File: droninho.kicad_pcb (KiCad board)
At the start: 2 copper layers, 26 x 49 mm, 19 parts, among them J1 M1, J2 M1, J3 M1, J4 M1, J5 Conn_01x02_Pin, Q1 SI2300, Q2 SI2300, Q3 SI2300, Q4 SI2300, U1 ESP32 Dev Kit, U2 MPU9250/6500

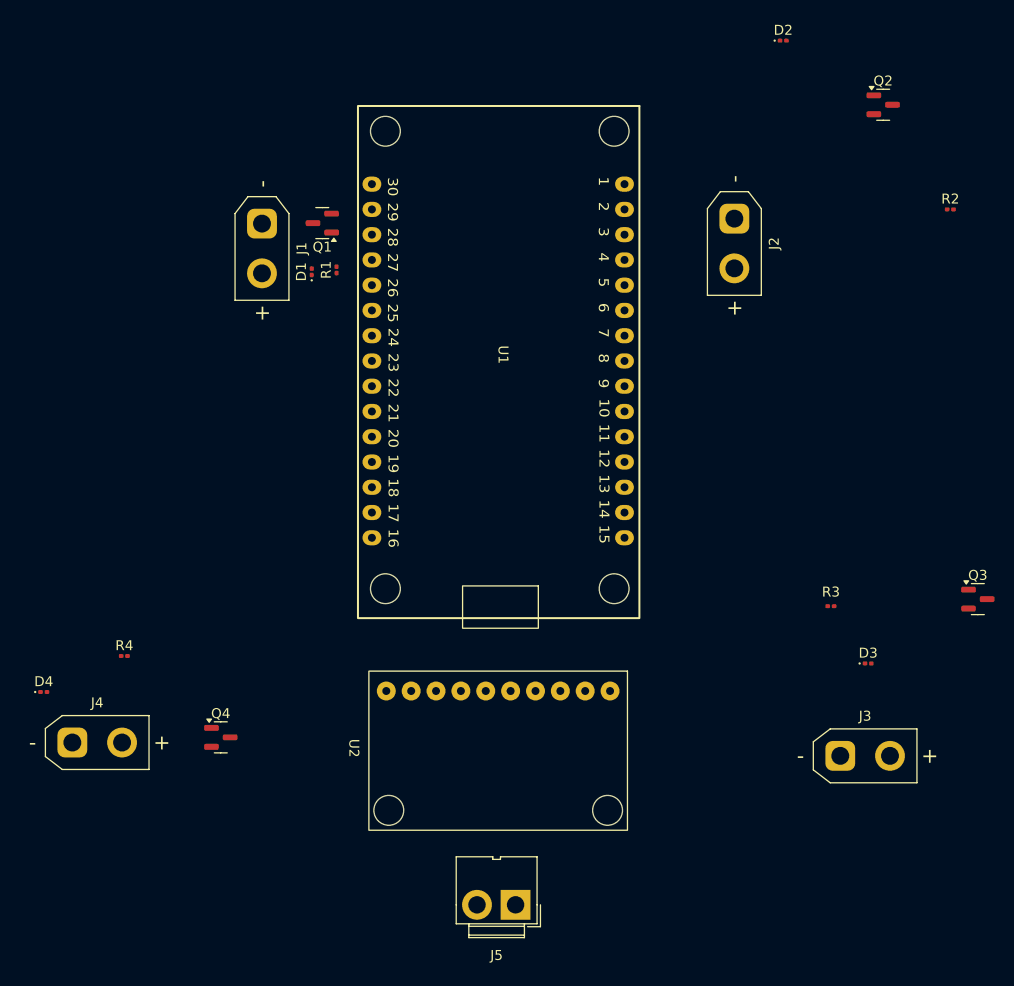
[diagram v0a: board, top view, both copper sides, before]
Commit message: Readme added
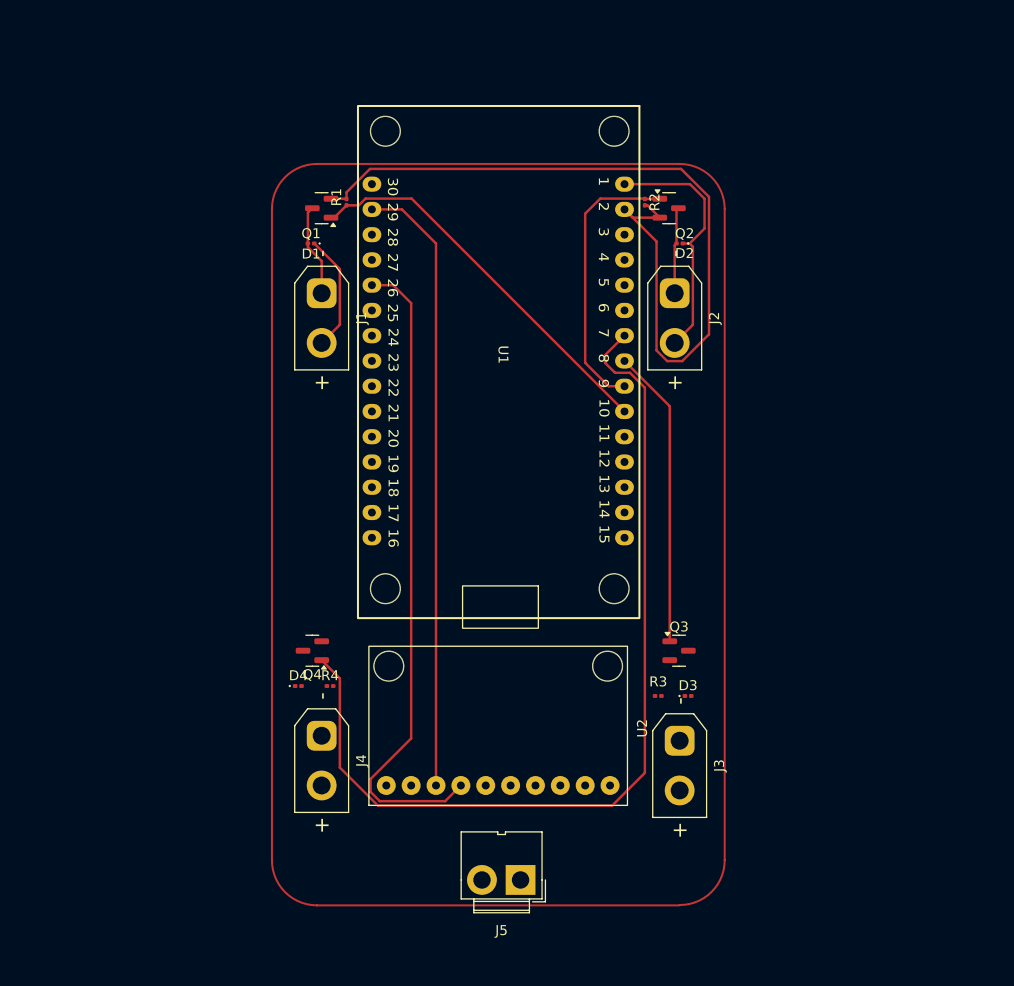
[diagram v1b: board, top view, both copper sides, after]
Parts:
- moved R2 30.7 mm to (148.5, 64.3), turned to -90 degrees
- moved Q3 30.5 mm to (151.9, 109.5)
- moved U2 29.3 mm to (120.8, 125.0), turned to 90 degrees
- moved D4 25.6 mm to (113.7, 113.0)
- moved J4 25.1 mm to (116.0, 118.0), turned to -90 degrees
- moved Q2 23.9 mm to (150.9, 65.0)
- moved D2 22.9 mm to (152.0, 68.5), turned to 180 degrees
- moved R4 20.9 mm to (116.8, 113.0)
- moved R3 19.6 mm to (149.8, 114.0)
- moved D3 18.4 mm to (152.8, 114.0)
- moved J3 16.2 mm to (152.0, 118.5), turned to -90 degrees
- moved Q4 12.7 mm to (115.1, 109.5), turned to 180 degrees
- moved J2 9.60 mm to (151.5, 73.5)
- moved J1 9.22 mm to (116.0, 73.5)
- moved R1 6.88 mm to (118.5, 64.3)
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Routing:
- net PWM4: track 0.00 -> 92.5 mm
- net GND: track 0.00 -> 82.9 mm
- net SDA: track 0.00 -> 65.7 mm
- net SCL: track 0.00 -> 62.4 mm
- net PWM1: track 0.00 -> 39.2 mm
- net +3.3V: track 0.00 -> 37.2 mm
- net PWM3: track 0.00 -> 30.1 mm
- net PWM2: track 0.00 -> 28.1 mm
- net Net-(D1-A): track 0.00 -> 9.31 mm
- net Net-(D2-A): track 0.00 -> 8.71 mm
